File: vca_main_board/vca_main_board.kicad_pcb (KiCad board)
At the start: 2 copper layers, 37 parts, among them J1 KPJX-4S-S, J2 Power terminal, Q1 STB15N80K5, Q2 STB15N80K5, SW1 POW_SWITCH, U1 173010335, U2 173010535, U3 173011235, U4 STM32H743VITx

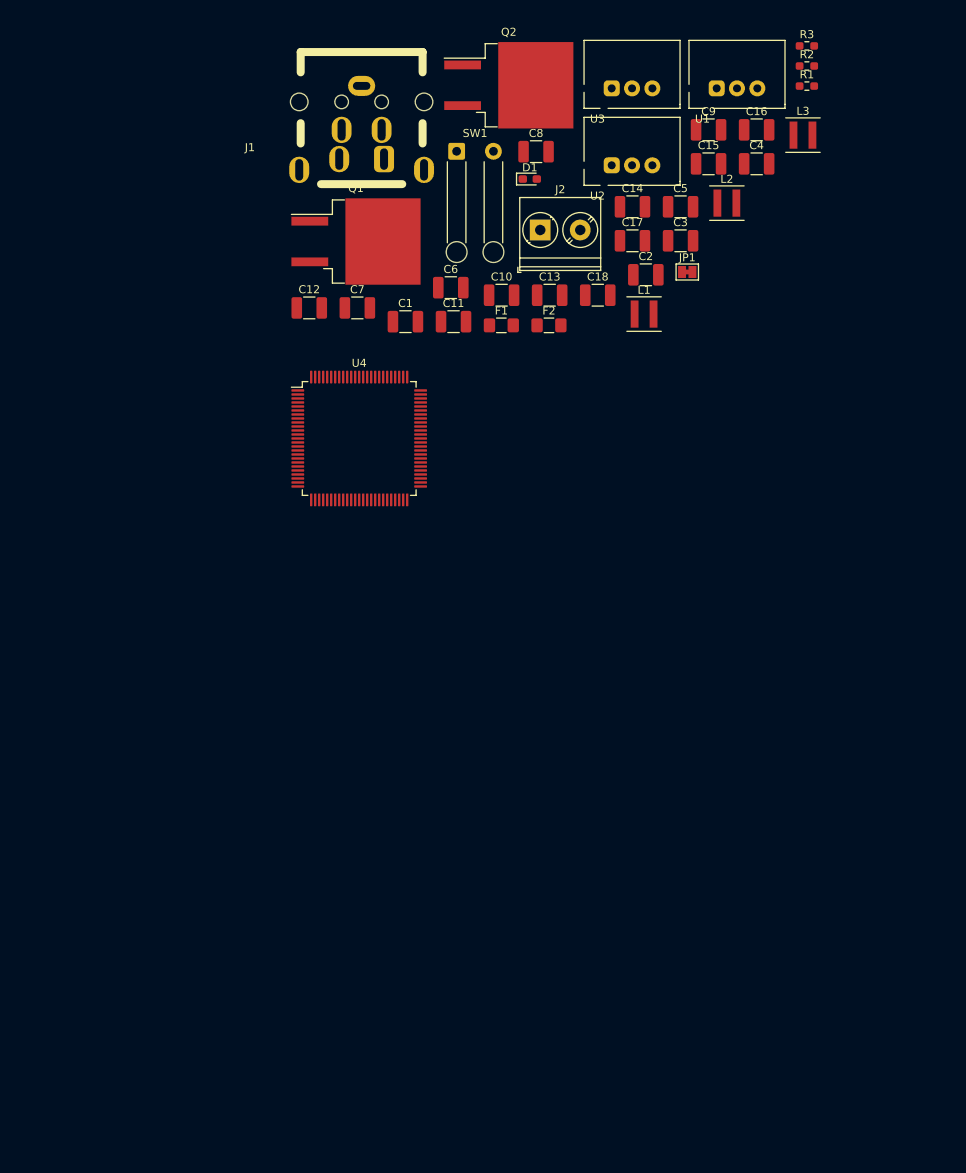
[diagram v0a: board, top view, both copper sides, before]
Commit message: done
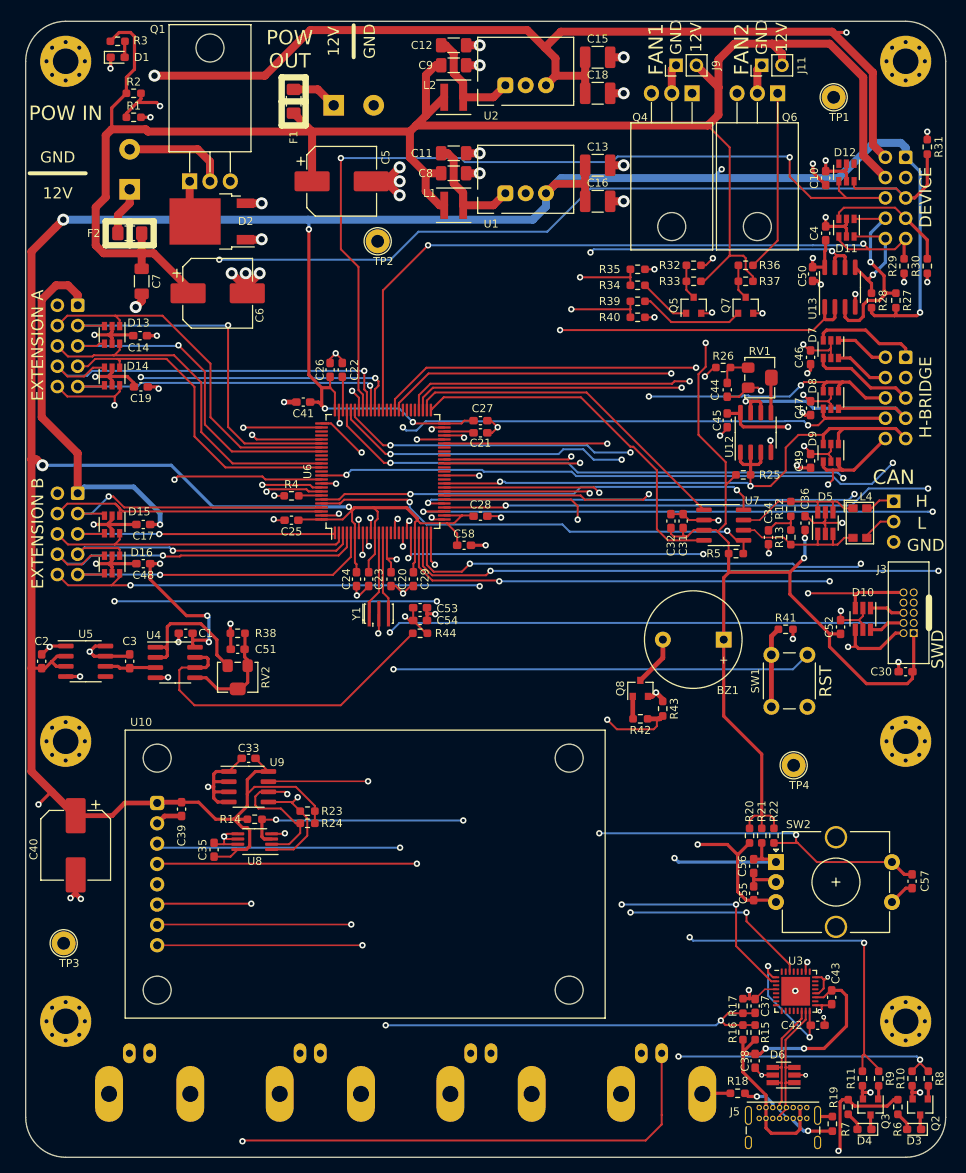
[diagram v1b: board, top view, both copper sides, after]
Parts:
- removed JP1: Jumper_NC, Jumper:SolderJumper-2_P1.3mm_Bridged_Pad1.0x1.5mm
- removed L3: XAL4030-472, Inductor_SMD:L_Coilcraft_XxL4030
- added BZ1: Buzzer, Buzzer_Beeper:Buzzer_12x9.5RM7.6, F.Cu at (117.2, 122.3)
- added C19: 100n 10V, Capacitor_SMD:C_0603_1608Metric_Pad1.08x0.95mm_HandSolder, F.Cu at (44.4, 90.7)
- added C20: 100n 6.3V, Capacitor_SMD:C_0603_1608Metric_Pad1.08x0.95mm_HandSolder, F.Cu at (75.7, 114.7)
- added C21: 2u2 6.3V, Capacitor_SMD:C_0603_1608Metric_Pad1.08x0.95mm_HandSolder, F.Cu at (86.8, 96.4)
- added C22: 2u2 6.3V, Capacitor_SMD:C_0603_1608Metric_Pad1.08x0.95mm_HandSolder, F.Cu at (69.6, 88.6)
- added C23: 100n 6.3V, Capacitor_SMD:C_0603_1608Metric_Pad1.08x0.95mm_HandSolder, F.Cu at (72.9, 114.7)
- added C24: 100n 6.3V, Capacitor_SMD:C_0603_1608Metric_Pad1.08x0.95mm_HandSolder, F.Cu at (71.4, 114.7)
- added C25: 100n 6.3V, Capacitor_SMD:C_0603_1608Metric_Pad1.08x0.95mm_HandSolder, F.Cu at (63.2, 107.4)
- added C26: 100n 6.3V, Capacitor_SMD:C_0603_1608Metric_Pad1.08x0.95mm_HandSolder, F.Cu at (68.0, 88.6)
- added C27: 100n 6.3V, Capacitor_SMD:C_0603_1608Metric_Pad1.08x0.95mm_HandSolder, F.Cu at (86.8, 94.9)
- added C28: 100n 6.3V, Capacitor_SMD:C_0603_1608Metric_Pad1.08x0.95mm_HandSolder, F.Cu at (86.8, 106.9)
- added C29: 100n 6.3V, Capacitor_SMD:C_0603_1608Metric_Pad1.08x0.95mm_HandSolder, F.Cu at (78.5, 114.7)
- added C30: 1u 6.3V, Capacitor_SMD:C_0603_1608Metric_Pad1.08x0.95mm_HandSolder, F.Cu at (140.0, 126.3)
- added C31: 100n 6.3V, Capacitor_SMD:C_0603_1608Metric_Pad1.08x0.95mm_HandSolder, F.Cu at (112.2, 107.5)
- added C32: 1u 6.3V, Capacitor_SMD:C_0603_1608Metric_Pad1.08x0.95mm_HandSolder, F.Cu at (110.7, 107.5)
- added C33: 100n 6.3V, Capacitor_SMD:C_0603_1608Metric_Pad1.08x0.95mm_HandSolder, F.Cu at (57.9, 137.1)
- added C34: 4n7 10V, Capacitor_SMD:C_0603_1608Metric_Pad1.08x0.95mm_HandSolder, F.Cu at (122.8, 109.5)
- added C35: 100n 6.3V, Capacitor_SMD:C_0603_1608Metric_Pad1.08x0.95mm_HandSolder, F.Cu at (53.5, 148.6)
- added C36: 1u 6.3V, Capacitor_SMD:C_0603_1608Metric_Pad1.08x0.95mm_HandSolder, F.Cu at (127.4, 107.7)
- added C37: 100n 10V, Capacitor_SMD:C_0603_1608Metric_Pad1.08x0.95mm_HandSolder, F.Cu at (121.2, 168.1)
- added C38: 100n 6.3V, Capacitor_SMD:C_0603_1608Metric_Pad1.08x0.95mm_HandSolder, F.Cu at (121.2, 174.9)
- added C39: 1u 6.3V, Capacitor_SMD:C_0603_1608Metric_Pad1.08x0.95mm_HandSolder, F.Cu at (49.5, 143.5)
- added C40: 180u 50V, Capacitor_SMD:CP_Elec_8x10.5, F.Cu at (36.2, 148.0)
- added C41: 4.7u 6.3V, Capacitor_SMD:C_0603_1608Metric_Pad1.08x0.95mm_HandSolder, F.Cu at (64.7, 92.6)
- added C42: 1u 6.3V, Capacitor_SMD:C_0603_1608Metric_Pad1.08x0.95mm_HandSolder, F.Cu at (129.0, 170.5)
- added C43: 1u 6.3V, Capacitor_SMD:C_0603_1608Metric_Pad1.08x0.95mm_HandSolder, F.Cu at (130.8, 167.0)
- added C44: 100n 6.3V, Capacitor_SMD:C_0603_1608Metric_Pad1.08x0.95mm_HandSolder, F.Cu at (117.7, 91.1)
- added C45: 100n 10V, Capacitor_SMD:C_0603_1608Metric_Pad1.08x0.95mm_HandSolder, F.Cu at (117.7, 94.9)
- added C46: 100n 10V, Capacitor_SMD:C_0603_1608Metric_Pad1.08x0.95mm_HandSolder, F.Cu at (128.1, 87.0)
- added C47: 100n 10V, Capacitor_SMD:C_0603_1608Metric_Pad1.08x0.95mm_HandSolder, F.Cu at (128.1, 93.4)
- added C48: 100n 10V, Capacitor_SMD:C_0603_1608Metric_Pad1.08x0.95mm_HandSolder, F.Cu at (44.7, 112.8)
- added C49: 100n 10V, Capacitor_SMD:C_0603_1608Metric_Pad1.08x0.95mm_HandSolder, F.Cu at (128.1, 100.0)
- added C50: 100n 10V, Capacitor_SMD:C_0603_1608Metric_Pad1.08x0.95mm_HandSolder, F.Cu at (128.4, 76.6)
- added C51: 100n 6.3V, Capacitor_SMD:C_0603_1608Metric_Pad1.08x0.95mm_HandSolder, F.Cu at (56.5, 123.5)
- added C52: 100n 6.3V, Capacitor_SMD:C_0603_1608Metric_Pad1.08x0.95mm_HandSolder, F.Cu at (131.9, 120.7)
- added C53: 1u 6.3V, Capacitor_SMD:C_0603_1608Metric_Pad1.08x0.95mm_HandSolder, F.Cu at (79.3, 118.3)
- added C54: 100n 6.3V, Capacitor_SMD:C_0603_1608Metric_Pad1.08x0.95mm_HandSolder, F.Cu at (79.3, 119.9)
- added C55: 100n 6.3V, Capacitor_SMD:C_0603_1608Metric_Pad1.08x0.95mm_HandSolder, F.Cu at (121.0, 154.0)
- added C56: 100n 6.3V, Capacitor_SMD:C_0603_1608Metric_Pad1.08x0.95mm_HandSolder, F.Cu at (121.0, 150.6)
- added C57: 100n 6.3V, Capacitor_SMD:C_0603_1608Metric_Pad1.08x0.95mm_HandSolder, F.Cu at (140.8, 152.5)
- added C58: 4.7u 6.3V, Capacitor_SMD:C_0603_1608Metric_Pad1.08x0.95mm_HandSolder, F.Cu at (84.8, 110.5)
- added D10: ESDA6V1BC6, Package_TO_SOT_SMD:SOT-23-6_Handsoldering, F.Cu at (134.7, 119.7)
- added D11: ESDA6V1BC6, Package_TO_SOT_SMD:SOT-23-6, F.Cu at (132.6, 70.8)
- added D12: ESDA6V1BC6, Package_TO_SOT_SMD:SOT-23-6, F.Cu at (132.6, 63.9)
- added D13: ESDA6V1BC6, Package_TO_SOT_SMD:SOT-23-6, F.Cu at (40.8, 84.2)
- added D14: ESDA6V1BC6, Package_TO_SOT_SMD:SOT-23-6, F.Cu at (40.8, 89.4)
- added D15: ESDA6V1BC6, Package_TO_SOT_SMD:SOT-23-6, F.Cu at (40.8, 107.9)
- added D16: ESDA6V1BC6, Package_TO_SOT_SMD:SOT-23-6, F.Cu at (40.8, 112.9)
- added D2: 10A 60V, Package_TO_SOT_SMD:TO-252-2, F.Cu at (53.3, 70.0)
- added D3: LED GREEN, LED_SMD:LED_0603_1608Metric_Pad1.05x0.95mm_HandSolder, F.Cu at (141.1, 183.5)
- added D4: LED GREEN, LED_SMD:LED_0603_1608Metric_Pad1.05x0.95mm_HandSolder, F.Cu at (134.8, 183.5)
- added D5: ESDA6V1BC6, Package_TO_SOT_SMD:SOT-23-6_Handsoldering, F.Cu at (130.0, 107.7)
- added D6: ESDA6V1BC6, Package_TO_SOT_SMD:SOT-23-6_Handsoldering, F.Cu at (124.7, 176.7)
- added D7: ESDA6V1BC6, Package_TO_SOT_SMD:SOT-23-6, F.Cu at (130.7, 86.0)
- added D8: ESDA6V1BC6, Package_TO_SOT_SMD:SOT-23-6, F.Cu at (130.7, 92.3)
- added D9: ESDA6V1BC6, Package_TO_SOT_SMD:SOT-23-6, F.Cu at (130.7, 98.9)
- added H1: Hole, MountingHole:MountingHole_3.2mm_M3_Pad_Via, F.Cu at (140.0, 170.0)
- added H2: Hole, MountingHole:MountingHole_3.2mm_M3_Pad_Via, F.Cu at (35.0, 170.0)
- added H3: Hole, MountingHole:MountingHole_3.2mm_M3_Pad_Via, F.Cu at (140.0, 135.0)
- added H4: Hole, MountingHole:MountingHole_3.2mm_M3_Pad_Via, F.Cu at (35.0, 135.0)
- added H5: Hole, MountingHole:MountingHole_3.2mm_M3_Pad_Via, F.Cu at (140.0, 50.0)
- added H6: Hole, MountingHole:MountingHole_3.2mm_M3_Pad_Via, F.Cu at (35.0, 50.0)
- added J10: IDC10, Connector_IDC:IDC-Header_2x05_P2.54mm_Vertical, B.Cu at (36.5, 80.5)
- added J11: Extra_fan_2, Connector_PinHeader_2.54mm:PinHeader_1x02_P2.54mm_Vertical, F.Cu at (122.0, 50.5)
- added J12: IDC10, Connector_IDC:IDC-Header_2x05_P2.54mm_Vertical, B.Cu at (36.5, 104.0)
- added J13: Conn_Coaxial, 1-1634613-0:1-1634613-0, B.Cu at (88.2, 174.0)
- added J14: Conn_Coaxial, 1-1634613-0:1-1634613-0, B.Cu at (66.8, 174.0)
- added J15: Conn_Coaxial, 1-1634613-0:1-1634613-0, B.Cu at (45.5, 174.0)
- added J3: SWD, 10pin_1.27_socket:10pin_1.27_socket, F.Cu at (141.0, 121.5)
- added J4: CAN, Connector_PinHeader_2.54mm:PinHeader_1x03_P2.54mm_Vertical, B.Cu at (138.5, 105.0)
- added J5: GCT USB4085, GCT_USB4085:USB_C_Receptacle_GCT_USB4085, F.Cu at (121.7, 180.8)
- added J6: IDC10, Connector_IDC:IDC-Header_2x05_P2.54mm_Vertical, B.Cu at (140.0, 87.0)
- added J7: Conn_Coaxial, 1-1634613-0:1-1634613-0, B.Cu at (109.5, 174.0)
- added J8: IDC10, Connector_IDC:IDC-Header_2x05_P2.54mm_Vertical, B.Cu at (140.0, 62.0)
- added J9: Extra_fan_1, Connector_PinHeader_2.54mm:PinHeader_1x02_P2.54mm_Vertical, F.Cu at (111.3, 50.5)
- added L4: PE-1812ACC101STS, Coilcraft_1812:L_CommonModeChoke_Coilcraft_1812CAN, F.Cu at (134.3, 107.7)
- added Q3: 2N7002, Package_TO_SOT_SMD:SOT-23, F.Cu at (135.6, 180.7)
- added Q4: IRF740, Package_TO_SOT_THT:TO-220-3_Horizontal_TabDown, F.Cu at (113.3, 54.0)
- added Q5: 2N7002, Package_TO_SOT_SMD:SOT-23, F.Cu at (113.5, 80.5)
- added Q6: IRF740, Package_TO_SOT_THT:TO-220-3_Horizontal_TabDown, F.Cu at (124.0, 54.0)
- added Q7: 2N7002, Package_TO_SOT_SMD:SOT-23, F.Cu at (120.0, 80.5)
- added Q8: 2N7002, Package_TO_SOT_SMD:SOT-23, F.Cu at (106.8, 128.4)
- added R10: 47k 5%, Resistor_SMD:R_0603_1608Metric_Pad0.98x0.95mm_HandSolder, F.Cu at (140.8, 177.2)
- added R11: 47k 5%, Resistor_SMD:R_0603_1608Metric_Pad0.98x0.95mm_HandSolder, F.Cu at (134.6, 177.2)
- added R12: 68R 1%, Resistor_SMD:R_0603_1608Metric_Pad0.98x0.95mm_HandSolder, F.Cu at (125.6, 105.9)
- added R13: 68R 1%, Resistor_SMD:R_0603_1608Metric_Pad0.98x0.95mm_HandSolder, F.Cu at (125.6, 109.5)
- added R14: 47k 5%, Resistor_SMD:R_0603_1608Metric_Pad0.98x0.95mm_HandSolder, F.Cu at (58.6, 144.7)
- added R15: 5k1 5%, Resistor_SMD:R_0603_1608Metric_Pad0.98x0.95mm_HandSolder, F.Cu at (121.2, 171.4)
- added R16: 5k1 5%, Resistor_SMD:R_0603_1608Metric_Pad0.98x0.95mm_HandSolder, F.Cu at (119.7, 171.4)
- added R17: 5k1 5%, Resistor_SMD:R_0603_1608Metric_Pad0.98x0.95mm_HandSolder, F.Cu at (119.7, 168.1)
- added R18: 5k1 5%, Resistor_SMD:R_0603_1608Metric_Pad0.98x0.95mm_HandSolder, F.Cu at (119.0, 179.0)
- added R19: 5k1 5%, Resistor_SMD:R_0603_1608Metric_Pad0.98x0.95mm_HandSolder, F.Cu at (130.8, 182.8)
- added R20: 47k 5%, Resistor_SMD:R_0603_1608Metric_Pad0.98x0.95mm_HandSolder, F.Cu at (120.5, 146.8)
- added R21: 47k 5%, Resistor_SMD:R_0603_1608Metric_Pad0.98x0.95mm_HandSolder, F.Cu at (122.0, 146.8)
- added R22: 47k 5%, Resistor_SMD:R_0603_1608Metric_Pad0.98x0.95mm_HandSolder, F.Cu at (123.5, 146.8)
- added R23: 2k2 5%, Resistor_SMD:R_0603_1608Metric_Pad0.98x0.95mm_HandSolder, F.Cu at (65.2, 143.7)
- added R24: 2k2 5%, Resistor_SMD:R_0603_1608Metric_Pad0.98x0.95mm_HandSolder, F.Cu at (65.2, 145.3)
- added R25: 10k 1%, Resistor_SMD:R_0603_1608Metric_Pad0.98x0.95mm_HandSolder, F.Cu at (119.7, 101.7)
- added R26: 5k1 1%, Resistor_SMD:R_0603_1608Metric_Pad0.98x0.95mm_HandSolder, F.Cu at (117.2, 88.3)
- added R27: 10k 1%, Resistor_SMD:R_0603_1608Metric_Pad0.98x0.95mm_HandSolder, F.Cu at (138.8, 79.9)
- added R28: 10k 1%, Resistor_SMD:R_0603_1608Metric_Pad0.98x0.95mm_HandSolder, F.Cu at (135.7, 79.9)
- added R29: 47k 5%, Resistor_SMD:R_0603_1608Metric_Pad0.98x0.95mm_HandSolder, F.Cu at (139.8, 75.6)
- added R30: 47k 5%, Resistor_SMD:R_0603_1608Metric_Pad0.98x0.95mm_HandSolder, F.Cu at (142.7, 75.6)
- added R31: 47k 5%, Resistor_SMD:R_0603_1608Metric_Pad0.98x0.95mm_HandSolder, F.Cu at (142.7, 60.7)
- added R32: 1k 5%, Resistor_SMD:R_0603_1608Metric_Pad0.98x0.95mm_HandSolder, F.Cu at (113.5, 75.5)
- added R33: 47k 5%, Resistor_SMD:R_0603_1608Metric_Pad0.98x0.95mm_HandSolder, F.Cu at (113.5, 77.5)
- added R34: 1k 5%, Resistor_SMD:R_0603_1608Metric_Pad0.98x0.95mm_HandSolder, F.Cu at (106.5, 78.0)
- added R35: 47k 5%, Resistor_SMD:R_0603_1608Metric_Pad0.98x0.95mm_HandSolder, F.Cu at (106.5, 76.0)
- added R36: 1k 5%, Resistor_SMD:R_0603_1608Metric_Pad0.98x0.95mm_HandSolder, F.Cu at (120.0, 75.5)
- added R37: 47k 5%, Resistor_SMD:R_0603_1608Metric_Pad0.98x0.95mm_HandSolder, F.Cu at (120.0, 77.5)
- added R38: 100k 1%, Resistor_SMD:R_0603_1608Metric_Pad0.98x0.95mm_HandSolder, F.Cu at (56.5, 121.5)
- added R39: 1k 5%, Resistor_SMD:R_0603_1608Metric_Pad0.98x0.95mm_HandSolder, F.Cu at (106.5, 80.0)
- added R4: 47k 5%, Resistor_SMD:R_0603_1608Metric_Pad0.98x0.95mm_HandSolder, F.Cu at (63.2, 104.3)
- added R40: 47k 5%, Resistor_SMD:R_0603_1608Metric_Pad0.98x0.95mm_HandSolder, F.Cu at (106.5, 82.0)
- added R41: 1k 5%, Resistor_SMD:R_0603_1608Metric_Pad0.98x0.95mm_HandSolder, F.Cu at (125.0, 121.0)
- added R42: 1k 5%, Resistor_SMD:R_0603_1608Metric_Pad0.98x0.95mm_HandSolder, F.Cu at (106.8, 132.2)
- added R43: 47k 5%, Resistor_SMD:R_0603_1608Metric_Pad0.98x0.95mm_HandSolder, F.Cu at (109.6, 130.9)
- added R44: 47R 1%, Resistor_SMD:R_0603_1608Metric_Pad0.98x0.95mm_HandSolder, F.Cu at (79.3, 121.5)
- added R5: 10k 5%, Resistor_SMD:R_0603_1608Metric_Pad0.98x0.95mm_HandSolder, F.Cu at (118.8, 111.5)
- added R6: 10k 5%, Resistor_SMD:R_0603_1608Metric_Pad0.98x0.95mm_HandSolder, F.Cu at (139.0, 180.7)
- added R7: 10k 5%, Resistor_SMD:R_0603_1608Metric_Pad0.98x0.95mm_HandSolder, F.Cu at (132.8, 180.7)
- added R8: 1k 5%, Resistor_SMD:R_0603_1608Metric_Pad0.98x0.95mm_HandSolder, F.Cu at (142.8, 177.2)
- added R9: 1k 5%, Resistor_SMD:R_0603_1608Metric_Pad0.98x0.95mm_HandSolder, F.Cu at (136.6, 177.2)
- added RV1: 10k, Bourns_3214W:Bourns_3214W, F.Cu at (121.8, 89.5)
- added RV2: 10k, Bourns_3214W:Bourns_3214W, F.Cu at (56.5, 127.0)
- added SW2: ALPS_EC12E, ALPS_EC12E:RotaryEncoder_Alps_EC12E-Switch_Vertical_H20mm_CircularMountingHoles, F.Cu at (123.8, 150.1)
- added TP1: GND, TestPoint:TestPoint_Loop_D2.60mm_Drill1.6mm_Beaded, F.Cu at (131.0, 54.5)
- added TP2: GND, TestPoint:TestPoint_Loop_D2.60mm_Drill1.6mm_Beaded, F.Cu at (74.0, 72.5)
- added TP3: GND, TestPoint:TestPoint_Loop_D2.60mm_Drill1.6mm_Beaded, F.Cu at (34.8, 160.2)
- added TP4: GND, TestPoint:TestPoint_Loop_D2.60mm_Drill1.6mm_Beaded, F.Cu at (126.0, 138.0)
- added U10: Waveshare_LCD_1_8, Waveshare_LCD_1.8:Waveshare_LCD_1.8, F.Cu at (46.4, 151.6)
- added U12: ADA4522-2ARZ, Package_SO:SOIC-8_3.9x4.9mm_P1.27mm, F.Cu at (121.3, 96.4)
- added U13: ADA4522-2ARZ, Package_SO:SOIC-8_3.9x4.9mm_P1.27mm, F.Cu at (131.8, 78.2)
- added U5: LM4140ACM-2.0, Package_SO:SOIC-8_3.9x4.9mm_P1.27mm, F.Cu at (37.5, 125.0)
- added U6: STM32H743VITx, Package_QFP:LQFP-100_14x14mm_P0.5mm, F.Cu at (74.7, 101.3)
- added U7: TCAN337, Package_SO:SOIC-8_3.9x4.9mm_P1.27mm, F.Cu at (117.3, 108.0)
- added U8: MCP9808_MSOP, Package_SO:MSOP-8_3x3mm_P0.65mm, F.Cu at (58.6, 147.5)
- added U9: M24256-BR, Package_SO:SOIC-8_3.9x4.9mm_P1.27mm, F.Cu at (57.9, 140.7)
- added Y1: 10MHz, Crystal:Resonator_SMD_muRata_CSTxExxV-3Pin_3.0x1.1mm_HandSoldering, F.Cu at (74.1, 119.1)
- C1: value 4u7/50V -> 1u 10V; footprint Capacitor_SMD:C_1210_3225Metric_Pad1.33x2.70mm_HandSolder -> Capacitor_SMD:C_0603_1608Metric_Pad1.08x0.95mm_HandSolder
- C10, C4: value 4u7/50V -> 100n 10V; footprint Capacitor_SMD:C_1210_3225Metric_Pad1.33x2.70mm_HandSolder -> Capacitor_SMD:C_0603_1608Metric_Pad1.08x0.95mm_HandSolder
- C11, C12, C7, C8, C9: value 4u7/50V -> 10u 20V; footprint Capacitor_SMD:C_1210_3225Metric_Pad1.33x2.70mm_HandSolder -> Capacitor_SMD:C_1206_3216Metric_Pad1.33x1.80mm_HandSolder
- C13, C15, C16, C18: value 22u/25V -> 22u 10V
- C14, C17: value 22u/25V -> 100n 10V; footprint Capacitor_SMD:C_1210_3225Metric_Pad1.33x2.70mm_HandSolder -> Capacitor_SMD:C_0603_1608Metric_Pad1.08x0.95mm_HandSolder
- C2, C3: value 4u7/50V -> 1u 6.3V; footprint Capacitor_SMD:C_1210_3225Metric_Pad1.33x2.70mm_HandSolder -> Capacitor_SMD:C_0603_1608Metric_Pad1.08x0.95mm_HandSolder
- C5, C6: value 4u7/50V -> 180u 50V; footprint Capacitor_SMD:C_1210_3225Metric_Pad1.33x2.70mm_HandSolder -> Capacitor_SMD:CP_Elec_8x10.5
- D1: value LED -> LED GREEN
- F1: value Fuse 4A -> Fuse 500mA
- F2: value Fuse 4A -> Fuse 1A
- J1: value KPJX-4S-S -> 12V_OUT; footprint KPJX-4S-S:KPJX-4S-S -> TerminalBlock_Phoenix:TerminalBlock_Phoenix_PT-1,5-2-5.0-H_1x02_P5.00mm_Horizontal; moved to B.Cu
- J2: value Power terminal -> 12V_IN; moved to B.Cu
- Q1: value STB15N80K5 -> IRF740; footprint Package_TO_SOT_SMD:TO-263-2 -> Package_TO_SOT_THT:TO-220-3_Horizontal_TabDown
- Q2: value STB15N80K5 -> 2N7002; footprint Package_TO_SOT_SMD:TO-263-2 -> Package_TO_SOT_SMD:SOT-23
- R1: value 100k 1% -> 47k 5%
- R2: value 100k 1% -> 100k 5%
- SW1: value POW_SWITCH -> RST; footprint Connector_Wire:SolderWire-0.5sqmm_1x02_P4.6mm_D0.9mm_OD2.1mm_Relief -> Button_Switch_THT:SW_PUSH_6mm_H4.3mm
- U3: value 173011235 -> FT232RQ; footprint 17301xx35:17301xx35 -> Package_DFN_QFN:QFN-32-1EP_5x5mm_P0.5mm_EP3.6x3.6mm
- U4: value STM32H743VITx -> ADA4522-2ARZ; footprint Package_QFP:LQFP-100_14x14mm_P0.5mm -> Package_SO:SOIC-8_3.9x4.9mm_P1.27mm
- moved Q2 137.7 mm to (141.8, 180.7), turned to 270 degrees
- moved U3 114.7 mm to (126.2, 166.2)
- moved C2 89.7 mm to (32.0, 125.0), turned to 90 degrees
- moved C3 86.6 mm to (43.0, 125.0), turned to 90 degrees
- moved R3 86.2 mm to (41.5, 47.5)
- moved R1 84.2 mm to (43.5, 57.0)
- moved R2 84.2 mm to (43.5, 54.0)
- moved SW1 79.8 mm to (123.2, 130.7), turned to 90 degrees
- moved C17 70.7 mm to (44.7, 107.9), turned to 180 degrees
- moved C14 63.6 mm to (44.3, 84.3), turned to 180 degrees
- moved D1 53.7 mm to (41.5, 49.5)
- moved F2 53.6 mm to (43.0, 71.5), turned to 180 degrees
- moved J2 51.6 mm to (43.0, 66.0), turned to 90 degrees
- moved C1 47.7 mm to (50.0, 121.5), turned to 180 degrees
- moved C10 43.1 mm to (130.0, 64.6), turned to 90 degrees
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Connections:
- C1 pad 1: +VDC -> +5V
- C10 pad 1: Net-(C10-Pad1) -> +5V
- C15 pad 1: +12V -> +5V
- C18 pad 1: +12V -> +5V
- C2 pad 1: +VDC -> +3V3
- C3 pad 1: +VDC -> Net-(C3-Pad1)
- C4 pad 1: +VDC -> +5V
- C5 pad 1: +VDC -> +12V
- C6 pad 1: +VDC -> +12V
- C7 pad 1: Net-(C10-Pad1) -> +12V
- C8 pad 1: Net-(C11-Pad1) -> +12V
- C9 pad 1: Net-(C12-Pad1) -> +12V
- F1 pad 1: Net-(F1-Pad1) -> +12V
- F2 pad 1: Net-(F1-Pad1) -> +12V
- J1 pad 1: Net-(J1-Pad1) -> Net-(F1-Pad2)
- J1 pad 2: Net-(F1-Pad2) -> GND
- J2 pad 1: Net-(J2-Pad1) -> Net-(F2-Pad2)
- J2 pad 2: Net-(F2-Pad2) -> Net-(J2-Pad2)
- L1 pad 1: +VDC -> +12V
- L1 pad 2: Net-(C10-Pad1) -> Net-(C11-Pad1)
- L2 pad 1: +VDC -> +12V
- L2 pad 2: Net-(C11-Pad1) -> Net-(C12-Pad1)
- Q1 pad 1: Net-(Q1-Pad1) -> Net-(D2-Pad2)
- Q1 pad 2: Net-(J1-Pad1) -> Net-(J2-Pad2)
- Q2 pad 2: Net-(J2-Pad1) -> GND
- Q2 pad 3: GND -> Net-(D3-Pad1)
- R1 pad 1: Net-(F1-Pad1) -> Net-(D2-Pad2)
- R1 pad 2: Net-(Q1-Pad1) -> GND
- R2 pad 1: Net-(F1-Pad1) -> +12V
- R2 pad 2: Net-(Q2-Pad1) -> Net-(D2-Pad2)
- R3 pad 1: +VDC -> +12V
- SW1 pad 1: Net-(F1-Pad1) -> Net-(R41-Pad1)
- SW1 pad 2: +VDC -> /MCU/NRST
- U1 pad 1: Net-(C10-Pad1) -> Net-(C11-Pad1)
- U2 pad 1: Net-(C11-Pad1) -> Net-(C12-Pad1)
- U3 pad 1: Net-(C12-Pad1) -> Net-(C42-Pad1)
- U3 pad 2: GND -> /MCU/USB_RX
- U3 pad 3: +12V -> (no net)
- U4 pad 1: Net-(U4-Pad1) -> Net-(RV2-Pad3)
- U4 pad 2: Net-(U4-Pad2) -> Net-(RV2-Pad3)
- U4 pad 3: Net-(U4-Pad3) -> Net-(C3-Pad1)
- U4 pad 4: Net-(U4-Pad4) -> GND
- U4 pad 6: Net-(U4-Pad6) -> Net-(R44-Pad1)
- U4 pad 7: Net-(U4-Pad7) -> Net-(R44-Pad1)
- U4 pad 8: Net-(U4-Pad8) -> +5V
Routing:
- net +3V3: track 0.00 -> 746.2 mm, vias 0 -> 13
- net +5V: track 0.00 -> 337.2 mm, vias 0 -> 14
- net /Mirror_Enc_A: track 0.00 -> 289.5 mm, vias 0 -> 3
- net GND: track 0.00 -> 288.3 mm, vias 0 -> 84
- net +12V: track 0.00 -> 238.8 mm
- net /Mirror_Enc_B: track 0.00 -> 191.5 mm, vias 0 -> 2
- net /MCU/LED_1: track 0.00 -> 151.9 mm, vias 0 -> 3
- net /MCU/LED_2: track 0.00 -> 147.0 mm, vias 0 -> 3
- net /MCU/USB_DET: track 0.00 -> 135.3 mm, vias 0 -> 3
- net /MCU/USB_RX: track 0.00 -> 119.5 mm, vias 0 -> 4
- net /GPIO_B: track 0.00 -> 119.0 mm, vias 0 -> 2
- net /MCU/USB_TX: track 0.00 -> 118.8 mm, vias 0 -> 4
- net /MCU/Knob_B: track 0.00 -> 118.2 mm, vias 0 -> 2
- net /MCU/Knob_A: track 0.00 -> 115.9 mm, vias 0 -> 2
- net /Coil_Fans: track 0.00 -> 107.2 mm, vias 0 -> 2
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- added copper zone on In1.Cu, net GND
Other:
- board outline added: 115 x 142 mm
- copper layers 2 -> 4
- board text added: "12V"
- board text added: "12V 2A"
- board text added: "12V 300mA"
- board text added: "CAN"
- board text added: "DEVICE"
- board text added: "EXTENSION A"
- board text added: "EXTENSION B"
- board text added: "FAN1"
- board text added: "FAN2"
- board text added: "GND"
- board text added: "H"
- board text added: "H-BRIDGE"
- board text added: "L"
- board text added: "POW IN"
- board text added: "POW OUT"
- board text added: "RST"
- board text added: "SWD"
